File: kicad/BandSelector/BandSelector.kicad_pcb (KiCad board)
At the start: 2 copper layers, 105.5 x 77.6 mm, 63 parts, among them J1 DE15_Plug_HighDensity_Mountin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, J2 POWER, J3 75915416LF, Q1 2N7000, Q2 2N7000, U1 PicoW, U2 L7805

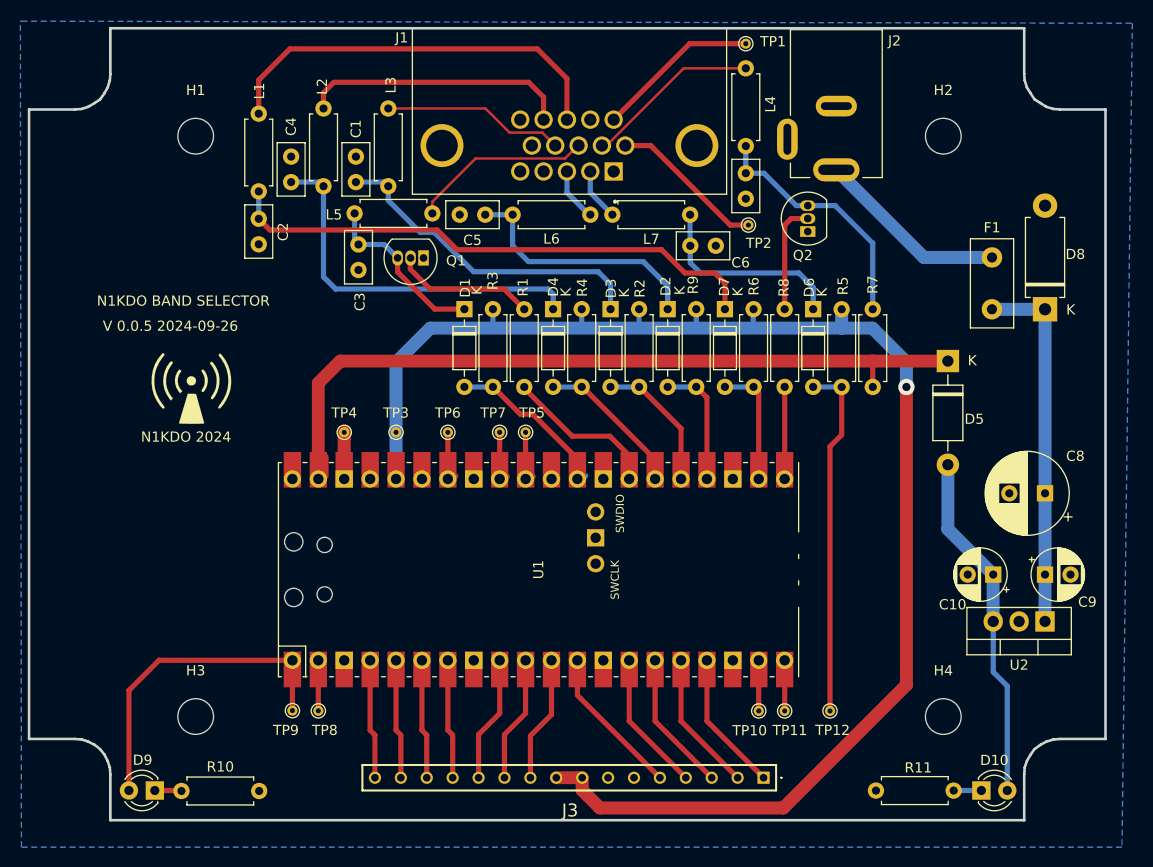
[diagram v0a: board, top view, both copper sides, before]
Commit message: software, meet hardware.
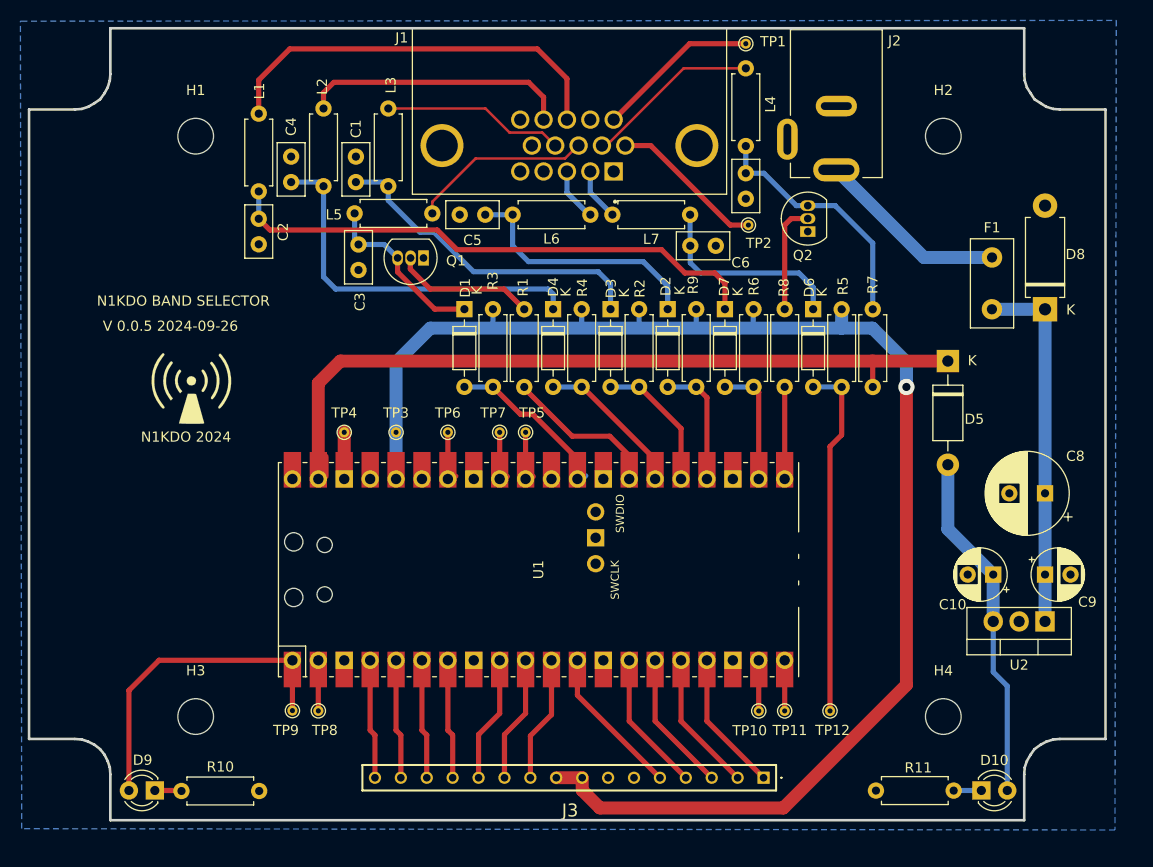
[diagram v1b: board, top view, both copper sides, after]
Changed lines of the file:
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@@
 			(layers "*.Cu" "*.Mask")
 			(remove_unused_layers no)
-			(net 6 "Net-(D1-K)")
+			(net 11 "Net-(D3-K)")
 			(pinfunction "2")
 			(pintype "passive")
@@
 			(layers "*.Cu" "*.Mask")
 			(remove_unused_layers no)
-			(net 11 "Net-(D3-K)")
+			(net 7 "Net-(D4-K)")
 			(pintype "passive")
 		)
@@
 			(layers "*.Cu" "*.Mask")
 			(remove_unused_layers no)
-			(net 9 "Net-(D2-K)")
+			(net 6 "Net-(D1-K)")
 			(pinfunction "K")
 			(pintype "passive")
@@
 			(layers "*.Cu" "*.Mask")
 			(remove_unused_layers no)
-			(net 9 "Net-(D2-K)")
+			(net 6 "Net-(D1-K)")
 			(pinfunction "D")
 			(pintype "passive")
@@
 			(layers "*.Cu" "*.Mask")
 			(remove_unused_layers no)
-			(net 6 "Net-(D1-K)")
+			(net 11 "Net-(D3-K)")
 			(pintype "passive")
 		)
@@
 			(layers "*.Cu" "*.Mask")
 			(remove_unused_layers no)
-			(net 7 "Net-(D4-K)")
+			(net 9 "Net-(D2-K)")
 			(pinfunction "2")
 			(pintype "passive")
@@
 			(layers "*.Cu" "*.Mask")
 			(remove_unused_layers no)
-			(net 6 "Net-(D1-K)")
+			(net 11 "Net-(D3-K)")
 			(pinfunction "K")
 			(pintype "passive")
@@
 			(layers "*.Cu" "*.Mask")
 			(remove_unused_layers no)
-			(net 9 "Net-(D2-K)")
+			(net 6 "Net-(D1-K)")
 			(pinfunction "2")
 			(pintype "passive")
@@
 			(layers "*.Cu" "*.Mask")
 			(remove_unused_layers no)
-			(net 9 "Net-(D2-K)")
+			(net 6 "Net-(D1-K)")
 			(pintype "passive")
 		)
@@
 			(layers "*.Cu" "*.Mask")
 			(remove_unused_layers no)
-			(net 7 "Net-(D4-K)")
+			(net 9 "Net-(D2-K)")
 			(pintype "passive")
 		)
@@
 			(layers "*.Cu" "*.Mask")
 			(remove_unused_layers no)
-			(net 11 "Net-(D3-K)")
+			(net 7 "Net-(D4-K)")
 			(pinfunction "K")
 			(pintype "passive")
@@
 			(layers "*.Cu" "*.Mask")
 			(remove_unused_layers no)
-			(net 11 "Net-(D3-K)")
+			(net 7 "Net-(D4-K)")
 			(pinfunction "2")
 			(pintype "passive")
@@
 			(layers "*.Cu" "*.Mask")
 			(remove_unused_layers no)
-			(net 7 "Net-(D4-K)")
+			(net 9 "Net-(D2-K)")
 			(pinfunction "K")
 			(pintype "passive")
@@
 	)
 	(segment
-		(start 156.92 77.04)
-		(end 156.92 77.47)
-		(width 0.508)
-		(layer "B.Cu")
-		(net 6)
-	)
-	(segment
-		(start 134.727 65.004)
-		(end 135.128 65.405)
-		(width 0.508)
-		(layer "B.Cu")
-		(net 6)
-	)
-	(segment
-		(start 156.92 75.005)
-		(end 155.702 73.787)
-		(width 0.508)
-		(layer "B.Cu")
-		(net 6)
-	)
-	(segment
-		(start 138.2395 69.9135)
-		(end 135.128 66.802)
+		(start 142.59 77.46)
+		(end 139.69 77.46)
 		(width 0.508)
-		(layer "B.Cu")
+		(layer "F.Cu")
 		(net 6)
 	)
 	(segment
-		(start 156.92 77.46)
-		(end 156.92 75.005)
+		(start 136.0424 73.8124)
+		(end 136.0424 72.4408)
 		(width 0.508)
-		(layer "B.Cu")
+		(layer "F.Cu")
 		(net 6)
 	)
 	(segment
-		(start 135.128 66.802)
-		(end 135.128 65.405)
+		(start 139.69 77.46)
+		(end 136.0424 73.8124)
 		(width 0.508)
-		(layer "B.Cu")
+		(layer "F.Cu")
 		(net 6)
 	)
 	(segment
-		(start 143.4846 73.787)
-		(end 139.6111 69.9135)
+		(start 131.826 70.739)
+		(end 132.207 71.12)
 		(width 0.508)
 		(layer "B.Cu")
@@
 	)
 	(segment
-		(start 131.953 65.004)
-		(end 134.727 65.004)
+		(start 131.826 68.072)
+		(end 131.826 70.739)
 		(width 0.508)
 		(layer "B.Cu")
@@
 	)
 	(segment
-		(start 139.6111 69.9135)
-		(end 138.2395 69.9135)
+		(start 134.7216 71.12)
+		(end 136.0424 72.4408)
 		(width 0.508)
 		(layer "B.Cu")
@@
 	)
 	(segment
-		(start 155.702 73.787)
-		(end 143.4846 73.787)
+		(start 132.207 71.12)
+		(end 134.7216 71.12)
 		(width 0.508)
 		(layer "B.Cu")
@@
 	)
 	(segment
-		(start 147.32 71.247)
-		(end 148.8694 72.7964)
+		(start 128.377 65.004)
+		(end 128.778 65.405)
 		(width 0.508)
 		(layer "B.Cu")
@@
 	)
 	(segment
-		(start 144.633 68.199)
-		(end 147.32 68.199)
+		(start 125.603 65.004)
+		(end 128.377 65.004)
 		(width 0.508)
 		(layer "B.Cu")
@@
 	)
 	(segment
-		(start 162.52 75.1948)
-		(end 162.52 77.46)
+		(start 150.7998 75.4888)
+		(end 129.9718 75.4888)
 		(width 0.508)
 		(layer "B.Cu")
@@
 	)
 	(segment
-		(start 147.32 68.199)
-		(end 147.32 71.247)
+		(start 151.29 75.979)
+		(end 150.7998 75.4888)
 		(width 0.508)
 		(layer "B.Cu")
@@
 	)
 	(segment
-		(start 162.52 77.13)
-		(end 162.52 77.47)
+		(start 128.778 74.295)
+		(end 128.778 65.405)
 		(width 0.508)
 		(layer "B.Cu")
@@
 	)
 	(segment
-		(start 148.8694 72.7964)
-		(end 160.1216 72.7964)
+		(start 129.9718 75.4888)
+		(end 128.778 74.295)
 		(width 0.508)
 		(layer "B.Cu")
@@
 	)
 	(segment
-		(start 160.1216 72.7964)
-		(end 162.52 75.1948)
+		(start 151.29 77.46)
+		(end 151.29 75.979)
 		(width 0.508)
 		(layer "B.Cu")
@@
 	)
 	(segment
-		(start 142.59 77.46)
-		(end 139.69 77.46)
+		(start 147.32 71.247)
+		(end 148.8694 72.7964)
 		(width 0.508)
-		(layer "F.Cu")
+		(layer "B.Cu")
 		(net 9)
 	)
 	(segment
-		(start 136.0424 73.8124)
-		(end 136.0424 72.4408)
+		(start 144.633 68.199)
+		(end 147.32 68.199)
 		(width 0.508)
-		(layer "F.Cu")
+		(layer "B.Cu")
 		(net 9)
 	)
 	(segment
-		(start 139.69 77.46)
-		(end 136.0424 73.8124)
+		(start 162.52 75.1948)
+		(end 162.52 77.46)
 		(width 0.508)
-		(layer "F.Cu")
+		(layer "B.Cu")
 		(net 9)
 	)
 	(segment
-		(start 131.826 70.739)
-		(end 132.207 71.12)
+		(start 147.32 68.199)
+		(end 147.32 71.247)
 		(width 0.508)
 		(layer "B.Cu")
@@
 	)
 	(segment
-		(start 131.826 68.072)
-		(end 131.826 70.739)
+		(start 162.52 77.13)
+		(end 162.52 77.47)
 		(width 0.508)
 		(layer "B.Cu")
@@
 	)
 	(segment
-		(start 134.7216 71.12)
-		(end 136.0424 72.4408)
+		(start 148.8694 72.7964)
+		(end 160.1216 72.7964)
 		(width 0.508)
 		(layer "B.Cu")
@@
 	)
 	(segment
-		(start 132.207 71.12)
-		(end 134.7216 71.12)
+		(start 160.1216 72.7964)
+		(end 162.52 75.1948)
 		(width 0.508)
 		(layer "B.Cu")
@@
 	)
 	(segment
-		(start 128.377 65.004)
-		(end 128.778 65.405)
+		(start 156.92 77.04)
+		(end 156.92 77.47)
 		(width 0.508)
 		(layer "B.Cu")
@@
 	)
 	(segment
-		(start 125.603 65.004)
-		(end 128.377 65.004)
+		(start 134.727 65.004)
+		(end 135.128 65.405)
 		(width 0.508)
 		(layer "B.Cu")
@@
 	)
 	(segment
-		(start 150.7998 75.4888)
-		(end 129.9718 75.4888)
+		(start 156.92 75.005)
+		(end 155.702 73.787)
 		(width 0.508)
 		(layer "B.Cu")
@@
 	)
 	(segment
-		(start 151.29 75.979)
-		(end 150.7998 75.4888)
+		(start 138.2395 69.9135)
+		(end 135.128 66.802)
 		(width 0.508)
 		(layer "B.Cu")
@@
 	)
 	(segment
-		(start 128.778 74.295)
-		(end 128.778 65.405)
+		(start 156.92 77.46)
+		(end 156.92 75.005)
 		(width 0.508)
 		(layer "B.Cu")
@@
 	)
 	(segment
-		(start 129.9718 75.4888)
-		(end 128.778 74.295)
+		(start 135.128 66.802)
+		(end 135.128 65.405)
 		(width 0.508)
 		(layer "B.Cu")
@@
 	)
 	(segment
-		(start 151.29 77.46)
-		(end 151.29 75.979)
+		(start 143.4846 73.787)
+		(end 139.6111 69.9135)
+		(width 0.508)
+		(layer "B.Cu")
+		(net 11)
+	)
+	(segment
+		(start 131.953 65.004)
+		(end 134.727 65.004)
+		(width 0.508)
+		(layer "B.Cu")
+		(net 11)
+	)
+	(segment
+		(start 139.6111 69.9135)
+		(end 138.2395 69.9135)
+		(width 0.508)
+		(layer "B.Cu")
+		(net 11)
+	)
+	(segment
+		(start 155.702 73.787)
+		(end 143.4846 73.787)
 		(width 0.508)
 		(layer "B.Cu")
@@
 		(polygon
 			(pts
-				(xy 99.1616 49.2252) (xy 208.0768 49.4284) (xy 207.0608 130.2004) (xy 99.1616 130.2004) (xy 99.06 49.2252)
+				(xy 99.1616 49.2252) (xy 206.502 49.149) (xy 206.375 128.524) (xy 99.187 128.397) (xy 99.06 49.2252)
 			)
 		)
